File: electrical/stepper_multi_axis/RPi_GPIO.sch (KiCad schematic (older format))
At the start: 6 parts, among them U10 Teensy4.1

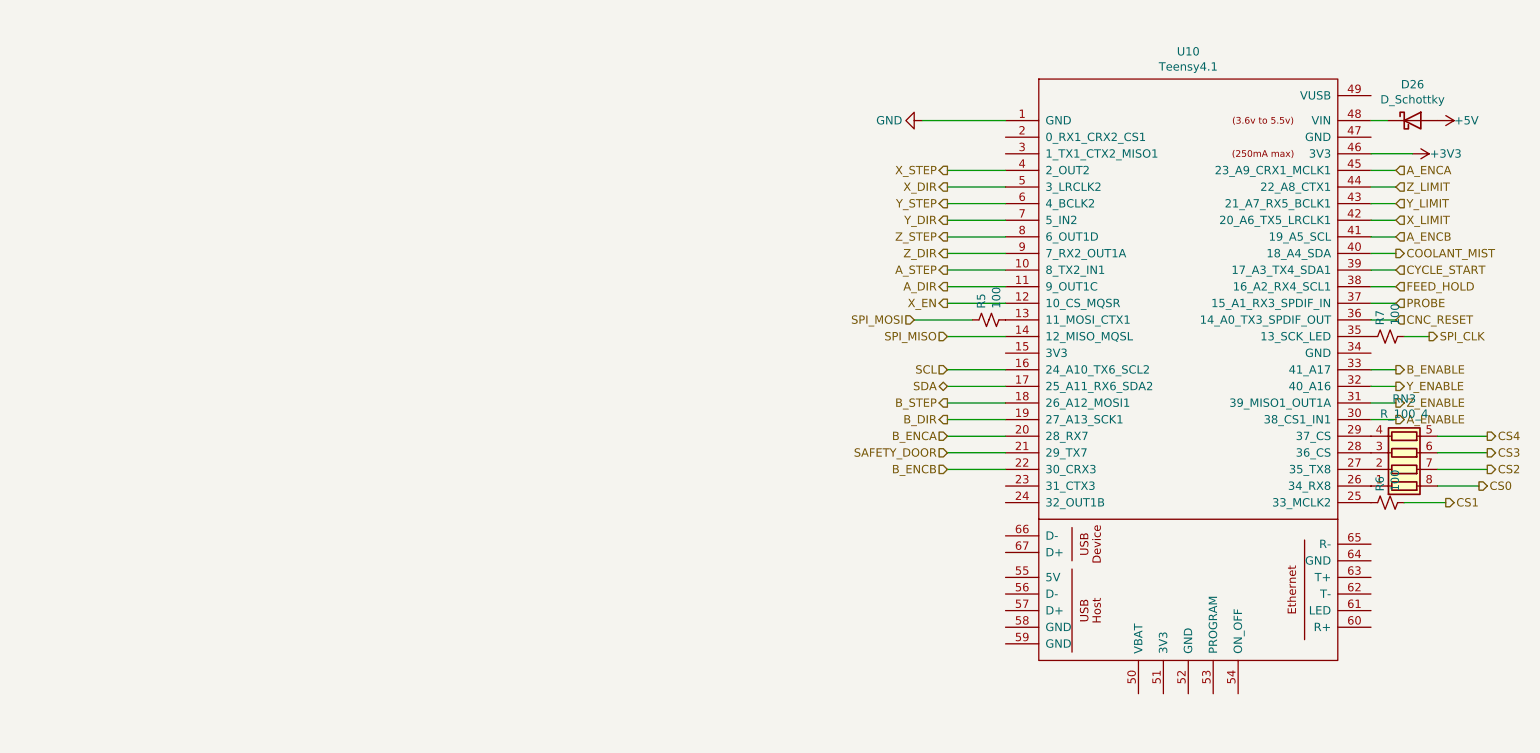
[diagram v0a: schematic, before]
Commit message: pre delete thru hole
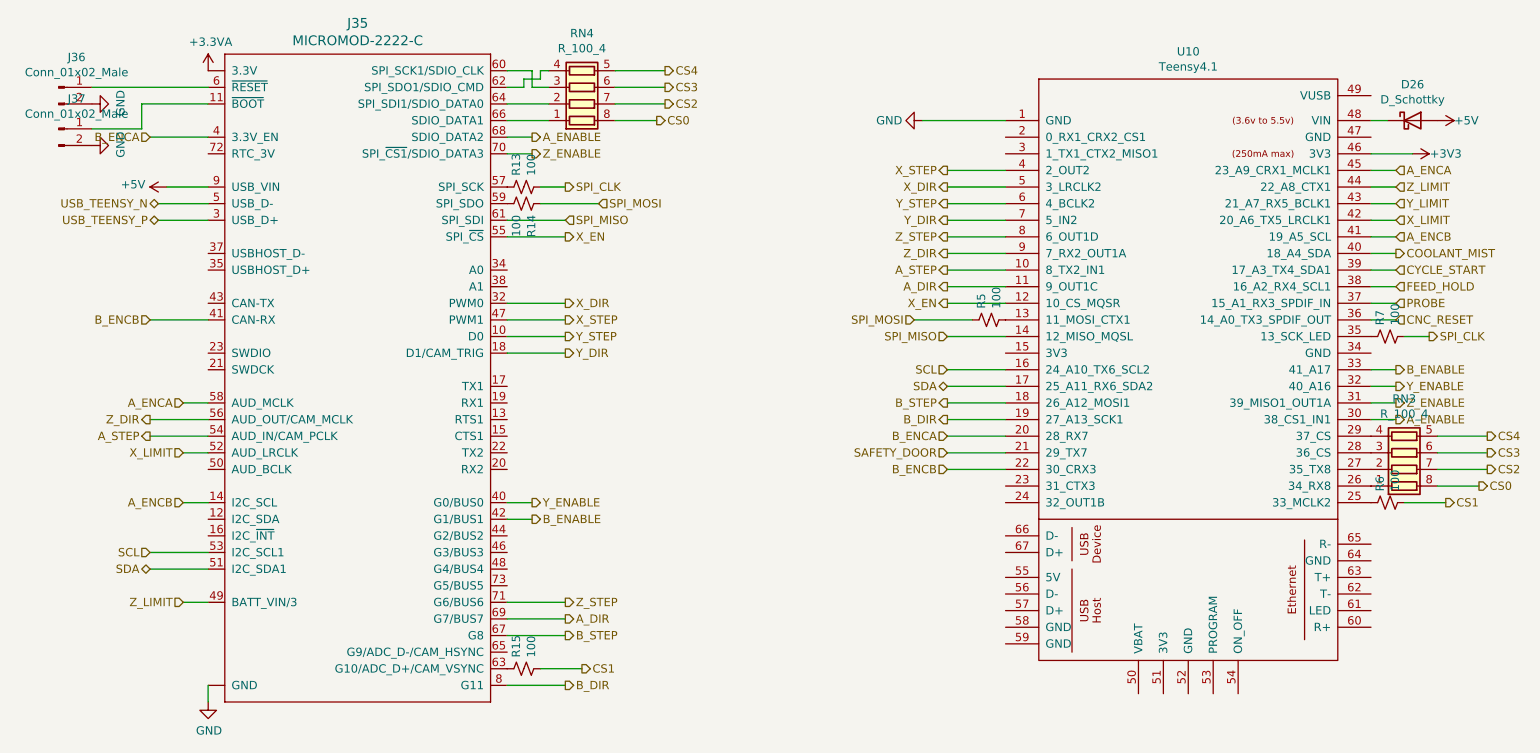
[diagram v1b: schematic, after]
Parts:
- added J35: MICROMOD-2222-C, SparkFun-MicroMod:M.2-CONNECTOR-E, symbol MicroMod_Processor_Board:MICROMOD-2222-C
- added J36, J37: Conn_01x02_Male, Connector_PinHeader_2.54mm:PinHeader_1x02_P2.54mm_Vertical, symbol Connector:Conn_01x02_Male
- added R13, R14, R15: 100, Resistor_SMD:R_0603_1608Metric_Pad0.98x0.95mm_HandSolder, symbol Device:R_Small_US
- added RN4: R_100_4, Resistor_SMD:R_Array_Concave_4x0603, symbol Device:R_Pack04
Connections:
- net +5V: now also J35.9 (USB_VIN)
- net A_DIR: now also J35.69 (G7/BUS7)
- net A_ENABLE: now also J35.68 (SDIO_DATA2)
- net A_ENCA: now also J35.58 (AUD_MCLK)
- net A_ENCB: now also J35.14 (I2C_SCL)
- net A_STEP: now also J35.54 (AUD_IN/CAM_PCLK)
- net B_DIR: now also J35.8 (G11)
- net B_ENABLE: now also J35.42 (G1/BUS1)
- net B_ENCA: now also J35.4 (3.3V_EN)
- net B_ENCB: now also J35.41 (CAN-RX)
- net B_STEP: now also J35.67 (G8)
- net CS0: now also RN4.8 (R1.2)
- net CS1: now also R15.2
- net CS2: now also RN4.7 (R2.2)
- net CS3: now also RN4.6 (R3.2)
- net CS4: now also RN4.5 (R4.2)
- net GND: now also J35.1 (GND), J35.33 (GND), J35.36 (GND), J35.39 (GND), J35.45 (GND), J35.7 (GND), J35.75 (GND), J36.2 (Pin_2), J37.2 (Pin_2)
- net SCL: now also J35.53 (I2C_SCL1)
- net SDA: now also J35.51 (I2C_SDA1)
- net SPI_CLK: now also R13.2
- net SPI_MISO: now also J35.61 (SPI_SDI)
- net SPI_MOSI: now also R14.1
- net X_DIR: now also J35.32 (PWM0)
- net X_EN: now also J35.55 (SPI_~CS~)
- net X_LIMIT: now also J35.52 (AUD_LRCLK)
- net X_STEP: now also J35.47 (PWM1)
- net Y_DIR: now also J35.18 (D1/CAM_TRIG)
- net Y_ENABLE: now also J35.40 (G0/BUS0)
- net Y_STEP: now also J35.10 (D0)
- net Z_DIR: now also J35.56 (AUD_OUT/CAM_MCLK)
- net Z_ENABLE: now also J35.70 (SPI_~CS1~/SDIO_DATA3)
- net Z_LIMIT: now also J35.49 (BATT_VIN/3)
- net Z_STEP: now also J35.71 (G6/BUS6)
- new net: J35.11 (~BOOT~), J37.1 (Pin_1)
- new net: J35.57 (SPI_SCK), R13.1
- new net: J35.59 (SPI_SDO), R14.2
- new net: J35.6 (~RESET~), J36.1 (Pin_1)
- new net: J35.60 (SPI_SCK1/SDIO_CLK), RN4.3 (R3.1)
- new net: J35.62 (SPI_SDO1/SDIO_CMD), RN4.4 (R4.1)
- new net: J35.63 (G10/ADC_D+/CAM_VSYNC), R15.1
- new net: J35.64 (SPI_SDI1/SDIO_DATA0), RN4.2 (R2.1)
- new net: J35.66 (SDIO_DATA1), RN4.1 (R1.1)
- new net +3.3VA: J35.2 (3.3V), J35.74 (3.3V)
- new net USB_TEENSY_N: J35.5 (USB_D-)
- new net USB_TEENSY_P: J35.3 (USB_D+)
